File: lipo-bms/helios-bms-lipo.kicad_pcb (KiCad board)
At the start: 4 copper layers, 34 x 19 mm, 66 parts, among them J1 Debug, J2 Output, J3 Outboard, J4 Battery, Q1 NMOS, Q2 SSM3J332R, U1 TPSM861253, U2 STM32L011F4Ux, U3 TPS22811, U4 TPS563207s, U5 BQ25306, U6 THVD1400D

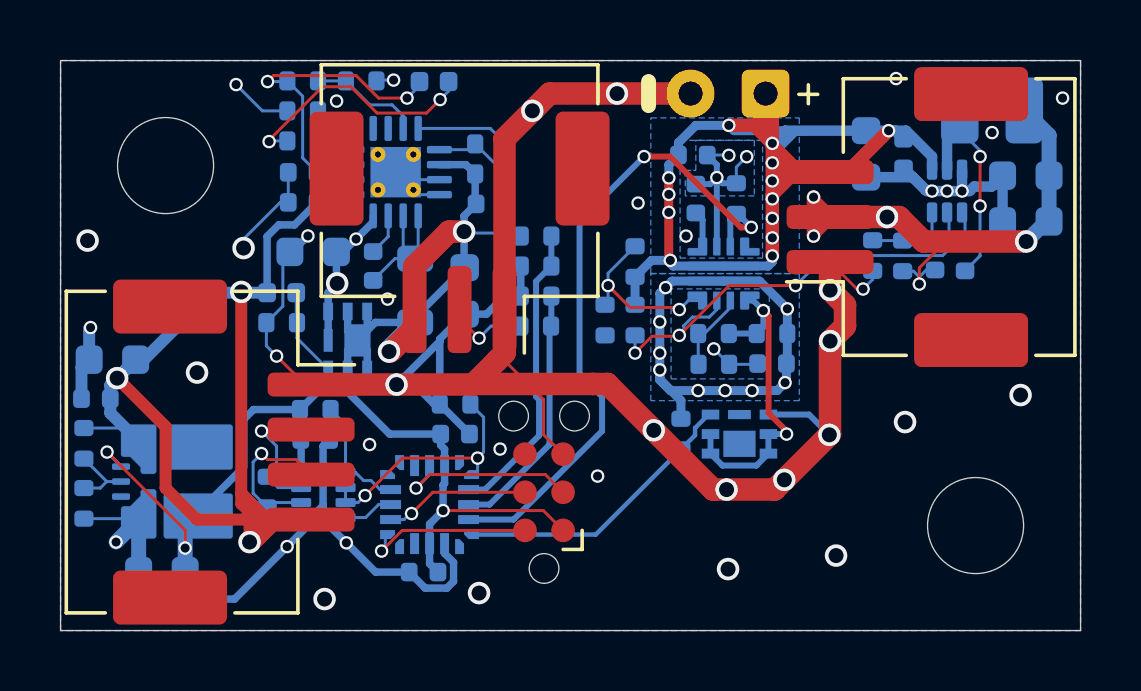
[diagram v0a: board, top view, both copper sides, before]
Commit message: satellite boards done
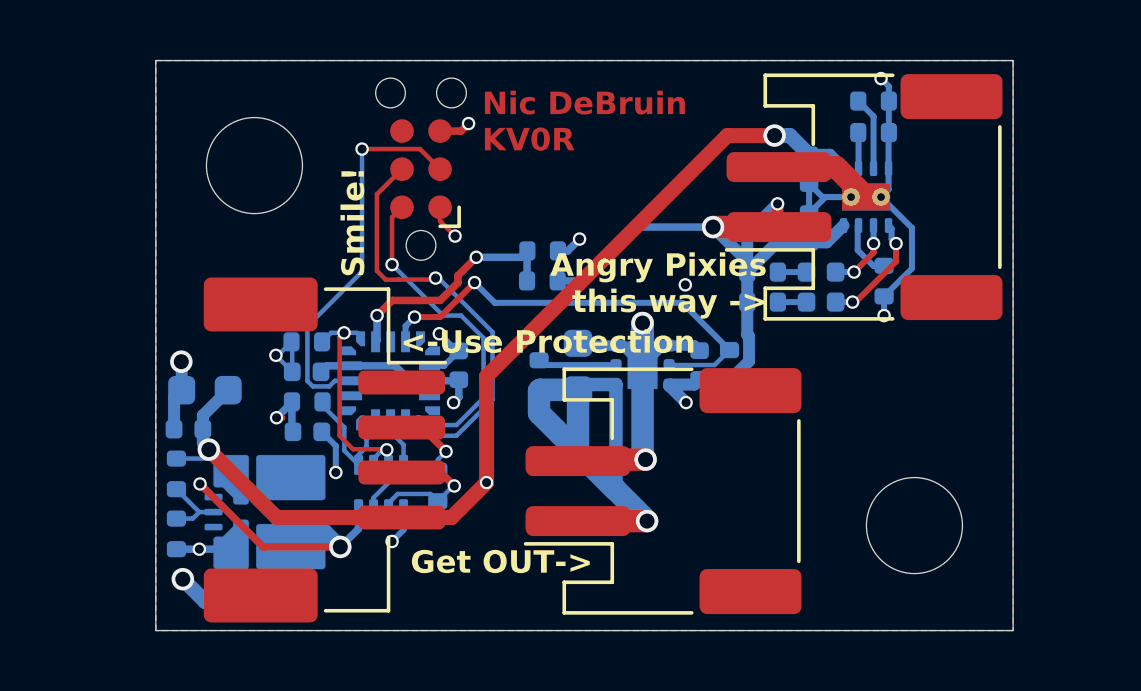
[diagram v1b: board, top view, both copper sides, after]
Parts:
- removed the C10 at (109.3, 73.6)
- removed C11: 470u, Capacitor_THT:CP_Radial_D6.3mm_P2.50mm
- removed C12, C15: 0.1u, Capacitor_SMD:C_0402_1005Metric
- removed C13, C14: 2.2u, Capacitor_SMD:C_0402_1005Metric
- removed C16: 22p, Capacitor_SMD:C_0402_1005Metric
- removed C17, C22: 10u, Capacitor_SMD:C_0603_1608Metric
- removed C18: 47n, Capacitor_SMD:C_0402_1005Metric
- removed C19, C21: 22u, Capacitor_SMD:C_0603_1608Metric
- removed C20: 470p, Capacitor_SMD:C_0402_1005Metric
- removed the C3 at (106.2, 80.6)
- removed the C9 at (103.6, 73.7)
- removed the J1 at (98.6, 84.9)
- removed L1: 3.3uH, Inductor_SMD:L_1008_2520Metric
- removed L2: 2.2uH, Inductor_SMD:L_0805_2012Metric
- removed Q1: NMOS, Helios-BMS:SOT-1220_UDFN6B_TOS-L
- removed Q2: SSM3J332R, Helios-BMS:SOT-1220_UDFN6B_TOS-L
- removed the R1 at (103.2, 83.0)
- removed the R10 at (101.7, 77.2)
- removed the R11 at (100.7, 79.2)
- removed R15: 36k, Resistor_SMD:R_0402_1005Metric
- removed R16, R17, R18: 10k, Resistor_SMD:R_0402_1005Metric
- removed R19: 1.1M, Resistor_SMD:R_0402_1005Metric
- removed R20: 200k, Resistor_SMD:R_0402_1005Metric
- removed R21, R25: 100k, Resistor_SMD:R_0402_1005Metric
- removed R26: 300k, Resistor_SMD:R_0402_1005Metric
- removed the R9 at (105.0, 75.1)
- removed the U4 at (112.0, 74.8)
- removed the U5 at (93.7, 74.2)
- added C4: 1u, Capacitor_SMD:C_0402_1005Metric, B.Cu at (107.5, 76.1)
- added C6: 1u, Capacitor_SMD:C_0402_1005Metric, B.Cu at (103.8, 80.7)
- added C7: 10u, Capacitor_SMD:C_0603_1608Metric, B.Cu at (99.8, 80.7)
- added J3: Output, Connector_JST:JST_PH_S2B-PH-SM4-TB_1x02-1MP_P2.00mm_Horizontal, F.Cu at (102.6, 84.8)
- added R3: 10k, Resistor_SMD:R_0402_1005Metric, B.Cu at (105.9, 78.5)
- added U2: BQ25176M, Package_SON:WSON-8-1EP_2x2mm_P0.5mm_EP0.9x1.6mm_ThermalVias, B.Cu at (109.3, 75.0)
- C5: value 1.5n -> 1u
- D2: value TBD -> PG; footprint Diode_SMD:D_0402_1005Metric -> LED_SMD:LED_0402_1005Metric
- J2: value Output -> Debug; footprint Connector_JST:JST_ZE_SM03B-ZESS-TB_1x03-1MP_P1.50mm_Horizontal -> Connector:Tag-Connect_TC2030-IDC-NL_2x03_P1.27mm_Vertical
- J4: footprint Connector_JST:JST_ZE_SM03B-ZESS-TB_1x03-1MP_P1.50mm_Horizontal -> Connector_JST:JST_PH_S2B-PH-SM4-TB_1x02-1MP_P2.00mm_Horizontal
- R12: value 10k -> 100k
- R13: value 160k -> 330k
- R14: value 300 -> TBD
- R4: value 430k -> 35.7k
- R5: value 100k -> 10k
- R6: value 51k -> 510R
- R7: value 500k -> 10k
- R8: value 300k -> 10k
- U3: value TPS22811 -> TPS22810DRV; footprint Helios-BMS:TPS22811 -> Package_SON:WSON-6-1EP_2x2mm_P0.65mm_EP1x1.6mm
- moved D2 18.0 mm to (107.8, 77.5)
- moved J2 16.3 mm to (94.5, 74.1)
- moved D1 14.8 mm to (107.8, 78.5)
- moved J4 13.6 mm to (109.3, 75.0), turned to 90 degrees
- moved R7 12.1 mm to (109.6, 71.8)
- moved R14 11.1 mm to (98.5, 81.0), turned to 90 degrees
- moved R6 9.38 mm to (109.6, 72.9)
- moved R13 9.26 mm to (98.6, 76.8), turned to 0 degrees
- moved R8 7.25 mm to (104.8, 80.7), turned to 90 degrees
- moved C9 6.99 mm to (95.8, 80.7), turned to 90 degrees
- moved R10 5.69 mm to (95.1, 84.7)
- moved C8 5.36 mm to (90.7, 80.9), turned to 180 degrees
- moved R11 5.36 mm to (90.7, 79.9)
- moved U4 4.32 mm to (93.5, 81.2), turned to 0 degrees
- moved R4 4.12 mm to (110.0, 77.8), turned to -90 degrees
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- renumbered C23 to C10, C8 to C3, C6 to C8, C4 to C9, J3 to J1, R2 to R1, R24 to R10, R23 to R11, R3 to R2, R22 to R9, U2 to U4, U6 to U5
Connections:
- C5 pad 1: Net-(U3-DV/DT) -> +12V
- D1 pad 2: /REGN -> Net-(D1-A)
- D2 pad 2: +12V -> Net-(D2-A)
- J2 pad 1: GND -> +3.3V
- J2 pad 2: +3V7 -> /SWDIO
- J2 pad 3: +VSW -> /~{RESET}
- J4 pad 1: GND -> +BATT
- J4 pad 2: /CENTER_TAP -> GND
- R12 pad 1: +VSW -> +BATT
- R12 pad 2: /SW_PG -> /PACK_ADC
- R13 pad 1: Net-(U5-ICHG) -> /PACK_ADC
- R14 pad 1: Net-(D1-K) -> +VSW
- R14 pad 2: Net-(U5-STAT) -> Net-(U3-QOD)
- R4 pad 1: VSYS -> Net-(U2-VSET)
- R4 pad 2: /EN/UVLO -> GND
- R5 pad 1: /EN/UVLO -> Net-(D2-A)
- R5 pad 2: /~{EN}/OVLO -> +BATT
- R6 pad 1: /~{EN}/OVLO -> Net-(U2-ISET)
- R7 pad 1: +BATT -> Net-(U2-BIAS)
- R7 pad 2: /PACK_ADC -> GND
- R8 pad 1: /PACK_ADC -> +BATT
- R8 pad 2: GND -> /GATE
- U3 pad 1: /EN/UVLO -> +VSW
- U3 pad 2: /~{EN}/OVLO -> Net-(U3-QOD)
- U3 pad 3: /SW_PG -> GND
- U3 pad 4: Net-(U3-PGTH) -> GND
- U3 pad 5: VSYS -> /GATE
- U3 pad 6: +VSW -> +BATT
- U3 pad 7: Net-(U3-DV/DT) -> GND
- U4 pad 10: /GATE -> unconnected-(U4-PA7-Pad10)
- U4 pad 8: /CENTER_TAP_ADC -> unconnected-(U4-PA5-Pad8)
- U4 pad 9: /IMON -> /GATE
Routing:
- net GND: track 118.1 -> 46.5 mm, vias 44 -> 14
- net +VSW: track 56.3 -> 19.6 mm, vias 13 -> 1
- net /IMON: track 22.4 -> 0.00 mm, vias 2 -> 0
- net VSYS: track 21.7 -> 0.00 mm, vias 11 -> 0
- net +3V7: track 21.2 -> 0.00 mm, vias 5 -> 0
- net /SW_PG: track 15.9 -> 0.00 mm, vias 3 -> 0
- net +BATT: track 22.4 -> 38.3 mm, vias 2 -> 3
- net +12V: track 40.0 -> 53.0 mm
- net /EN/UVLO: track 11.2 -> 0.00 mm, vias 2 -> 0
- net /REGN: track 10.9 -> 0.00 mm, vias 2 -> 0
- net /SWCLK: track 4.86 -> 14.5 mm
- net /CENTER_TAP_ADC: track 8.50 -> 0.00 mm
- net Net-(U4-SW): track 7.99 -> 0.00 mm, vias 2 -> 0
- net +3.3V: track 31.1 -> 38.5 mm, vias 3 -> 5
- net /~{RESET}: track 6.27 -> 13.0 mm
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- added copper zone on In2.Cu, net GND
- removed copper zone on In2.Cu, net +12V
- removed copper zone on In2.Cu, net +3V7
- removed copper zone on B.Cu, net +VSW
- removed copper zone on In2.Cu, net +VSW
- removed copper zone on B.Cu, net VSYS
- removed copper zone on In2.Cu, net VSYS
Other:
- board size 34 x 19 mm -> 28.6 x 19 mm
- board text added: "1S LiPo BMS Satellite Project Helios 2026"
- board text added: "<-Use Protection"
- board text added: "Angry Pixies this way ->"
- board text added: "Design change made in time."
- board text added: "Get OUT->"
- board text added: "Nic DeBruin KV0R"
- board text added: "Smile!"
- board text added: "Tasty tasty AA's"
